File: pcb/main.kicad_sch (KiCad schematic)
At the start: 1 part

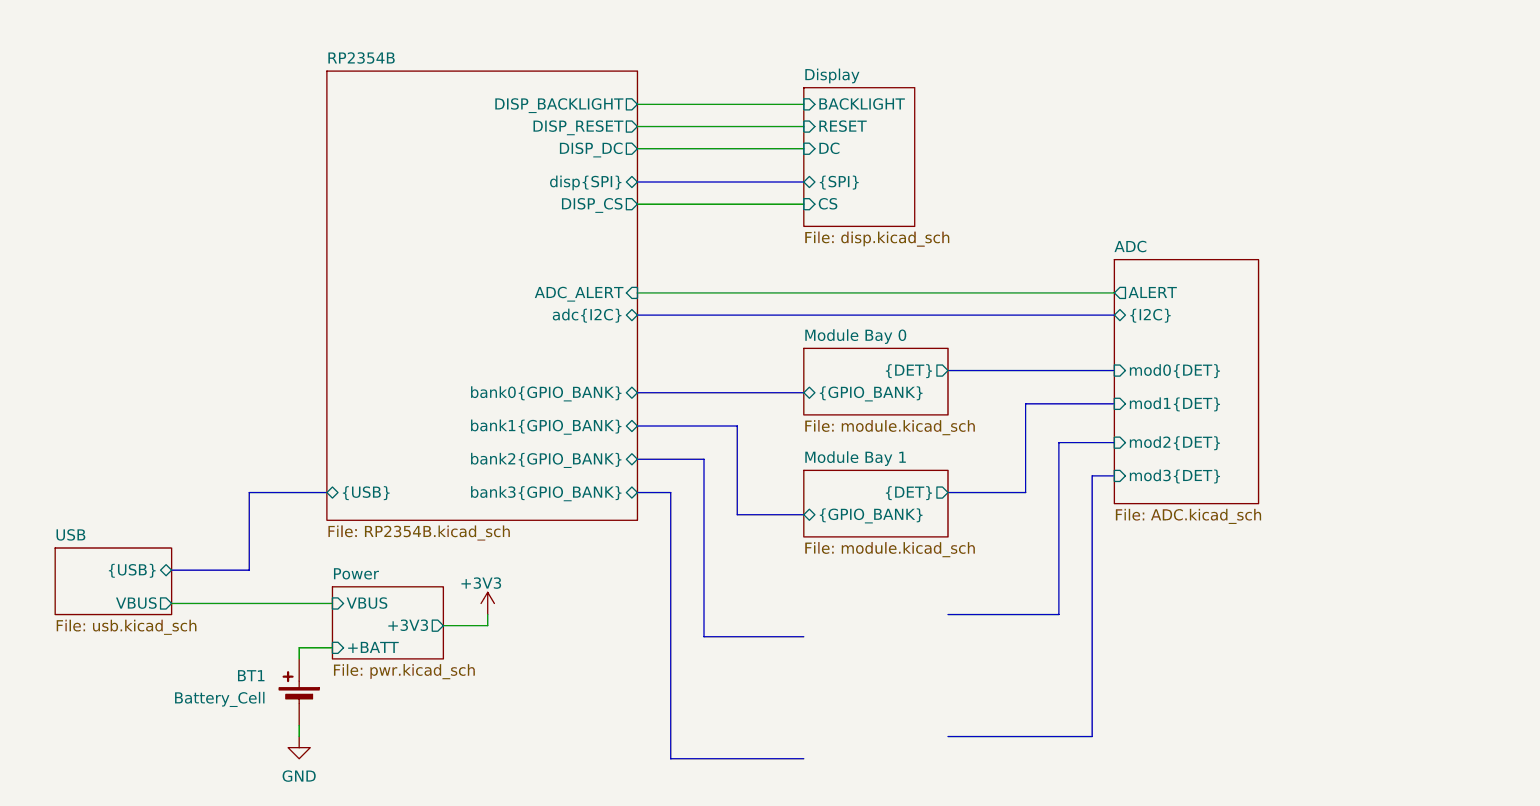
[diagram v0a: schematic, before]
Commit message: moved stuff around
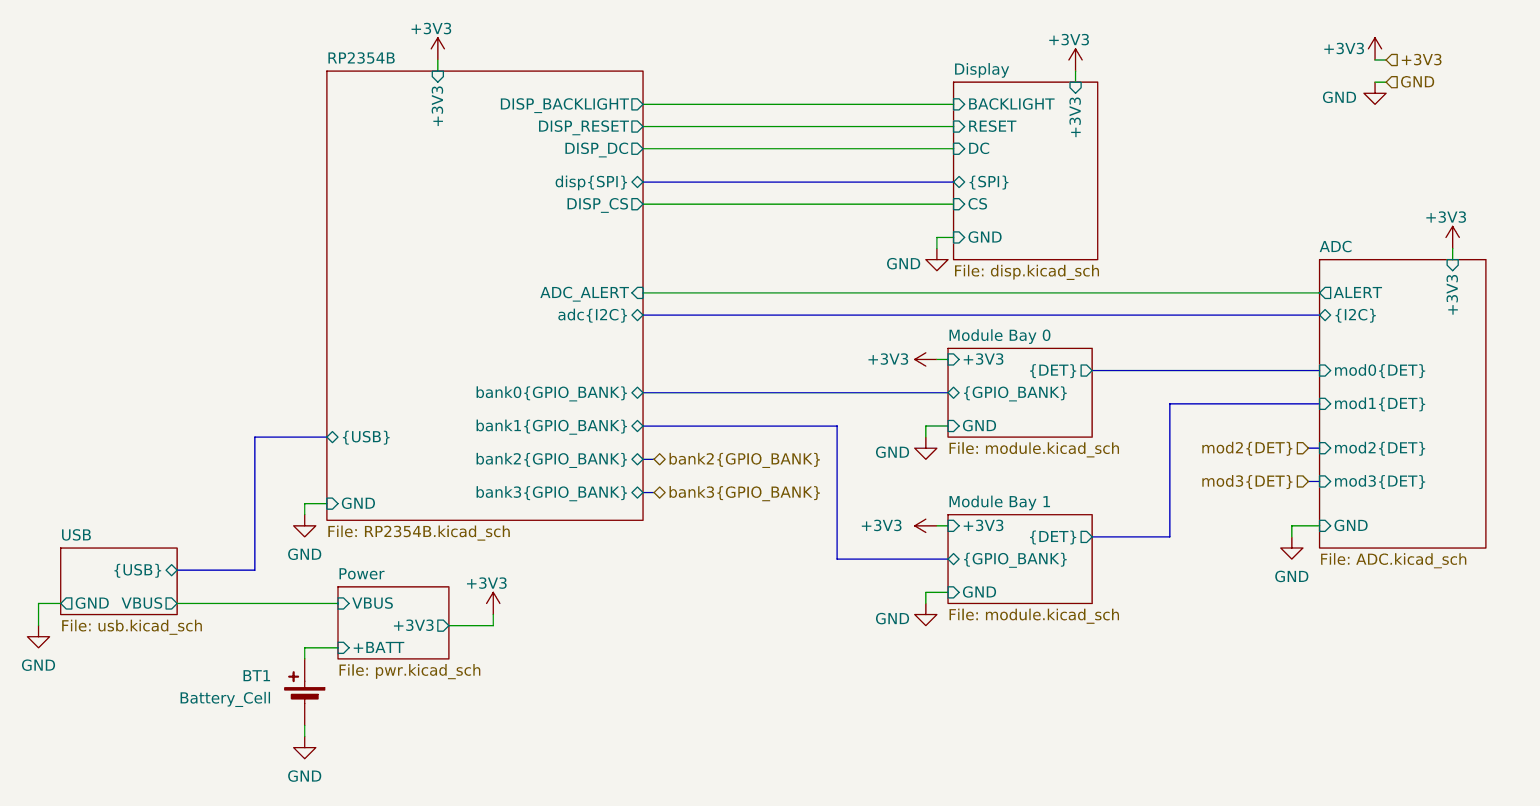
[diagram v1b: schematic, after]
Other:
- sheet ADC ports: added +3V3, GND; removed none
- sheet Display ports: added +3V3, GND; removed none
- sheet Module Bay 0 ports: added +3V3, GND; removed none
- sheet Module Bay 1 ports: added +3V3, GND; removed none
- sheet RP2354B ports: added +3V3, GND; removed none
- sheet USB ports: added GND; removed none
- moved on the sheet: BT1

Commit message: did some layout
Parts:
- BT1: footprint Connector_JST:JST_PH_S2B-PH-SM4-TB_1x02-1MP_P2.00mm_Horizontal -> Connector_Molex:Molex_PicoBlade_53261-0271_1x02-1MP_P1.25mm_Horizontal
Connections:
- net GND: now also BT1.1 (-); no longer BT1.2 (-)
- net Power/+BATT: now also BT1.2 (+); no longer BT1.1 (+)
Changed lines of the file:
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@@
 			)
 		)
-		(property "Footprint" "Connector_JST:JST_PH_S2B-PH-SM4-TB_1x02-1MP_P2.00mm_Horizontal"
+		(property "Footprint" "Connector_Molex:Molex_PicoBlade_53261-0271_1x02-1MP_P1.25mm_Horizontal"
 			(at 107.315 121.666 90)
 			(hide yes)
